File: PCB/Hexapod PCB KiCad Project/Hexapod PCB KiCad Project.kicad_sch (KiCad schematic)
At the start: 3 parts, among them J1 Male Pin Header 1x3, J2 Power Terminal, U1 DEV-16771

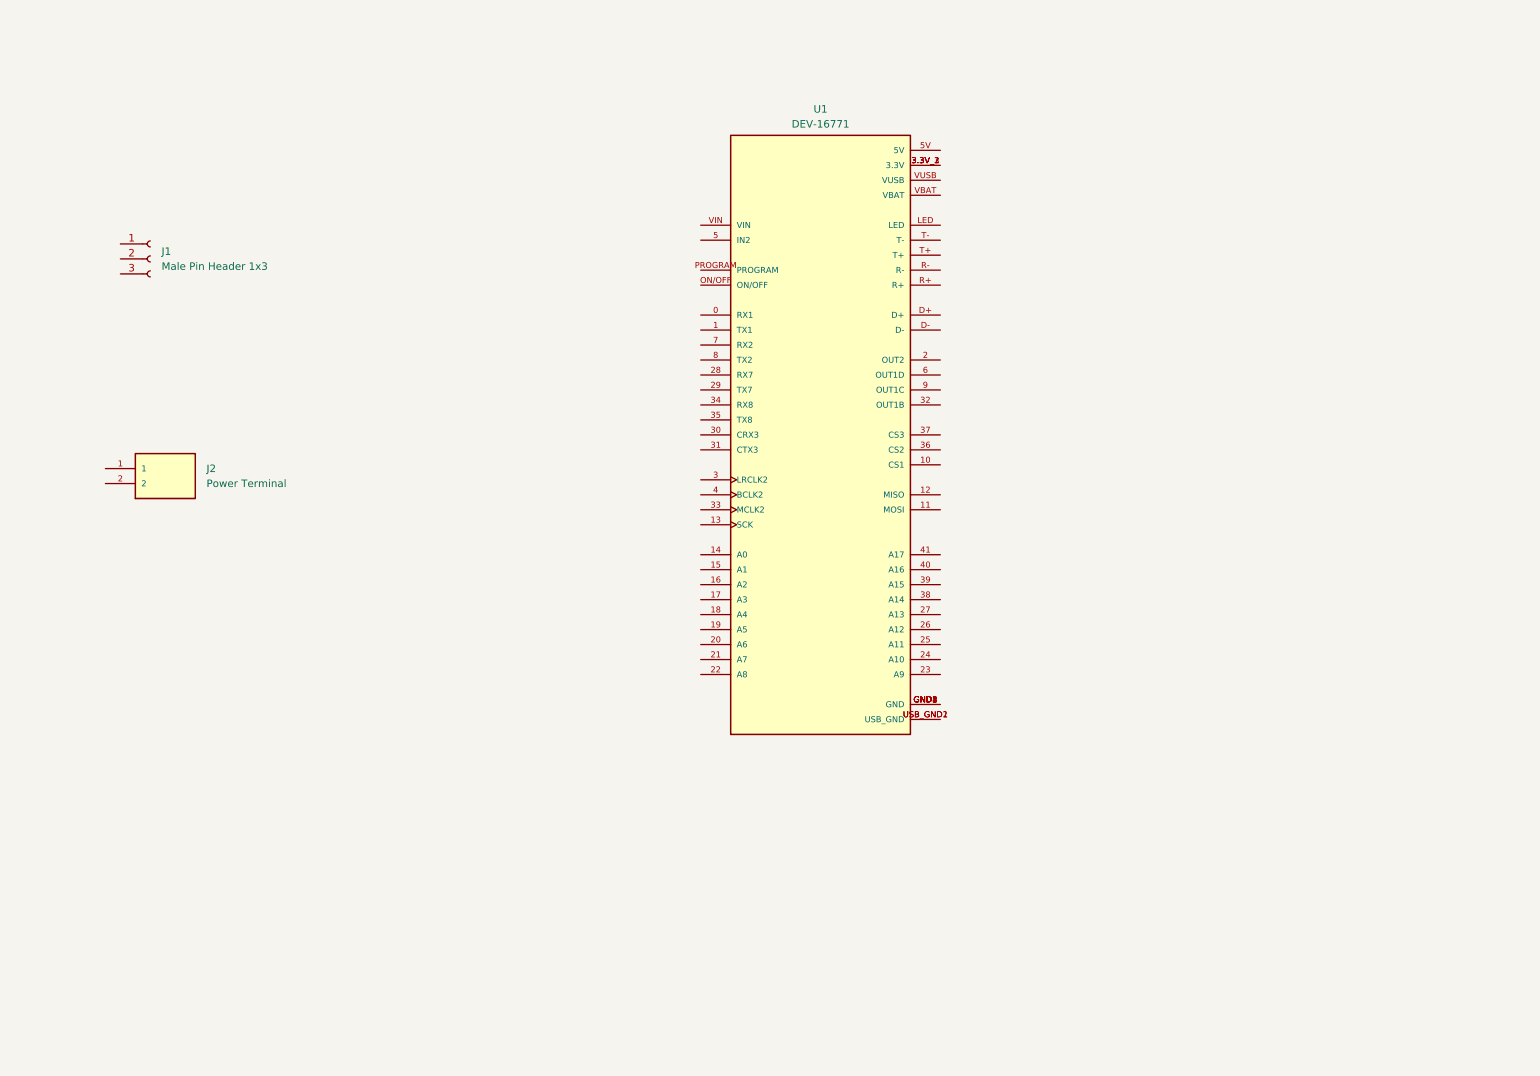
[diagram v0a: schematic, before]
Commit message: Pcb updates
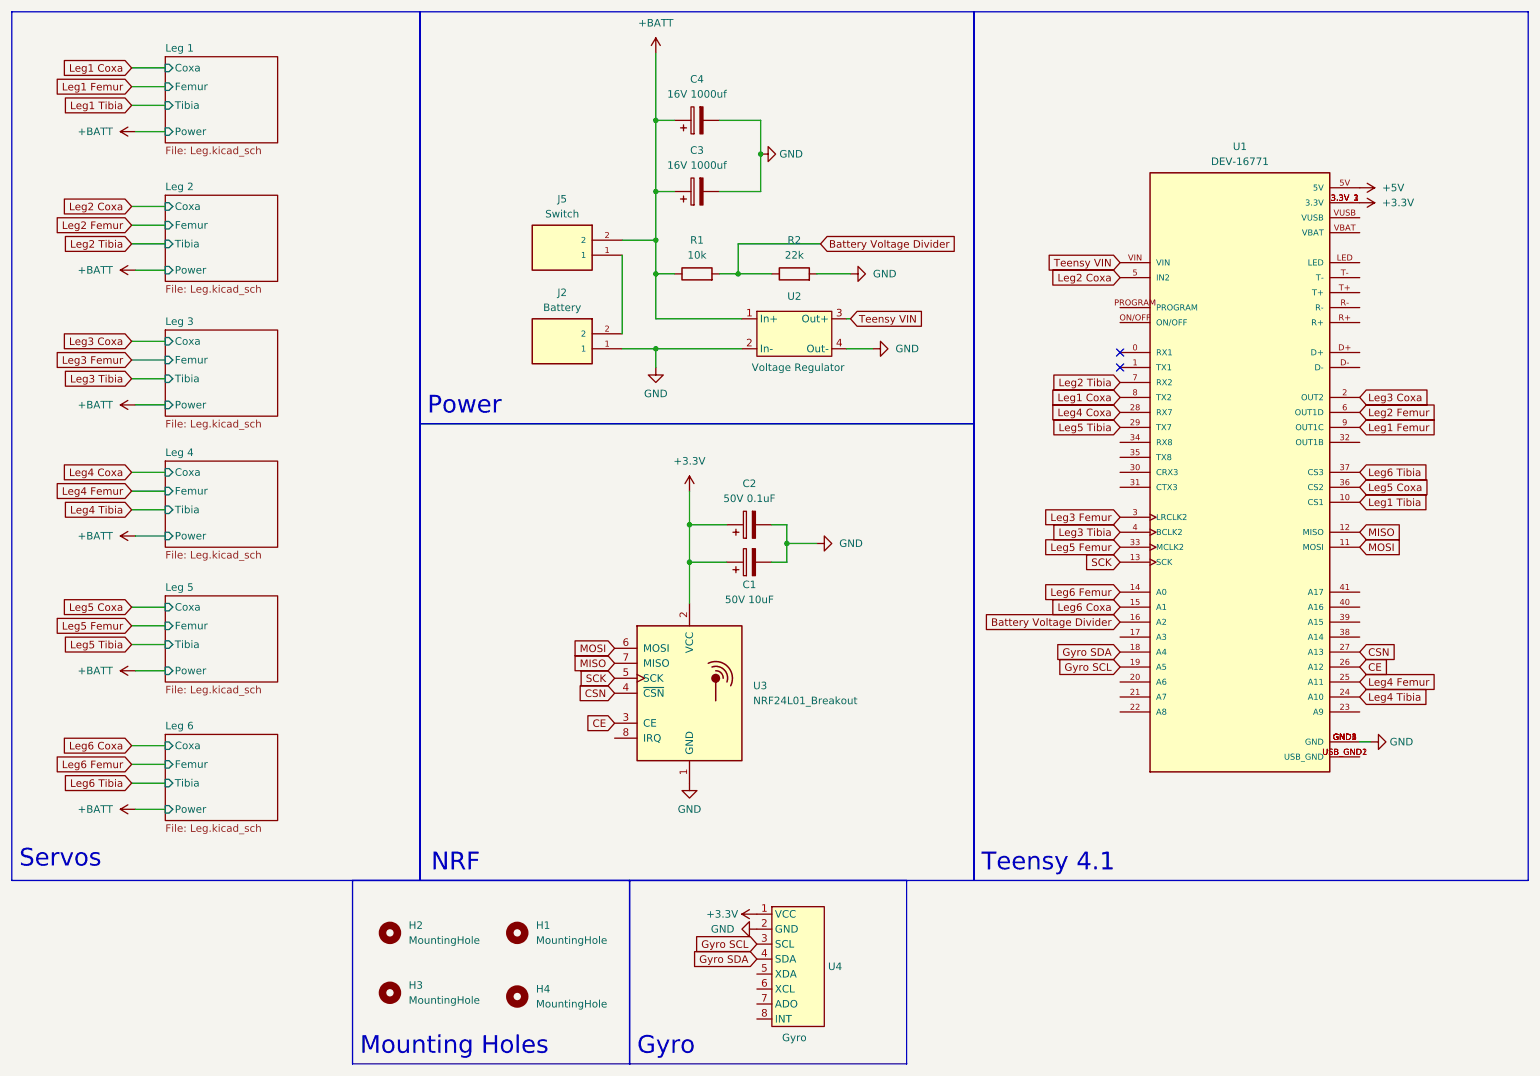
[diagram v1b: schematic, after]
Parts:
- removed J1: Male Pin Header 1x3, Connector_PinHeader_2.54mm:PinHeader_1x03_P2.54mm_Vertical, symbol Connector:Conn_01x03_Socket
- removed J2: Power Terminal, Terminal 2 Pin:CUI_TB005-762-02BE, symbol Terminal 2 Pin:TB005-762-02BE
- removed U1: DEV-16771, TEENSY 4.1:MODULE_DEV-16771, symbol TEENSY 4.1:DEV-16771
- added C1: 50V 10uF, Capacitor_THT:CP_Radial_D5.0mm_P2.00mm, symbol Device:C_Polarized
- added C2: 50V 0.1uF, Capacitor_THT:CP_Radial_D4.0mm_P2.00mm, symbol Device:C_Polarized
- added C3, C4: 16V 1000uf, Capacitor_THT:CP_Radial_D10.0mm_P5.00mm, symbol Device:C_Polarized
- added H1, H2, H3, H4: MountingHole, MountingHole:MountingHole_3.2mm_M3, symbol Mechanical:MountingHole
- added J2: Battery, Terminal 2 Pin:CUI_TB005-762-02BE, symbol Power Terminal 2 Pin:TB005-762-02BE
- added J5: Switch, Terminal 2 Pin:CUI_TB005-762-02BE, symbol Power Terminal 2 Pin:TB005-762-02BE
- added R1: 10k, Resistor_THT:R_Axial_DIN0207_L6.3mm_D2.5mm_P7.62mm_Horizontal, symbol Device:R
- added R2: 22k, Resistor_THT:R_Axial_DIN0207_L6.3mm_D2.5mm_P7.62mm_Horizontal, symbol Device:R
- added U1: DEV-16771, Teensy 4.1:MODULE_DEV-16771, symbol Teensy 4.1:DEV-16771
- added U2: Voltage Regulator, Voltage Regulator LM2596:Voltage Regulator LM2596, symbol Voltage Regulator LM2596:Voltage_Regulator_LM2596
- added U3: NRF24L01_Breakout, RF_Module:nRF24L01_Breakout, symbol RF:NRF24L01_Breakout
- added U4: Gyro, MPU6050 THT:MPU6050 THT, symbol MPU6050 THT:MPU6050_THT
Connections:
- new net: U1.USB_GND1 (USB_GND), U1.USB_GND2 (USB_GND)
- new net: J2.2, J5.1
- new net +3.3V: C1.1, C2.1, U1.3.3V_1 (3.3V), U1.3.3V_2 (3.3V), U1.3.3V_3 (3.3V), U3.2 (VCC), U4.1 (VCC)
- new net +5V: U1.5V
- new net +BATT: C3.1, C4.1, J5.2, R1.1, U2.1 (In+)
- new net Battery Voltage Divider: R1.2, R2.1, U1.16 (A2)
- new net CE: U1.26 (A12), U3.3 (CE)
- new net CSN: U1.27 (A13), U3.4 (~{CSN})
- new net GND: C1.2, C2.2, C3.2, C4.2, J2.1, R2.2, U1.GND1 (GND), U1.GND2 (GND), U1.GND3 (GND), U1.GND4 (GND), U1.GND5 (GND), U2.2 (In-), U2.4 (Out-), U3.1 (GND), U4.2 (GND)
- new net Gyro SCL: U1.19 (A5), U4.3 (SCL)
- new net Gyro SDA: U1.18 (A4), U4.4 (SDA)
- new net Leg1 Coxa: U1.8 (TX2)
- new net Leg1 Femur: U1.9 (OUT1C)
- new net Leg1 Tibia: U1.10 (CS1)
- new net Leg2 Coxa: U1.5 (IN2)
- new net Leg2 Femur: U1.6 (OUT1D)
- new net Leg2 Tibia: U1.7 (RX2)
- new net Leg3 Coxa: U1.2 (OUT2)
- new net Leg3 Femur: U1.3 (LRCLK2)
- new net Leg3 Tibia: U1.4 (BCLK2)
- new net Leg4 Coxa: U1.28 (RX7)
- new net Leg4 Femur: U1.25 (A11)
- new net Leg4 Tibia: U1.24 (A10)
- new net Leg5 Coxa: U1.36 (CS2)
- new net Leg5 Femur: U1.33 (MCLK2)
- new net Leg5 Tibia: U1.29 (TX7)
- new net Leg6 Coxa: U1.15 (A1)
- new net Leg6 Femur: U1.14 (A0)
- new net Leg6 Tibia: U1.37 (CS3)
- new net MISO: U1.12 (MISO), U3.7 (MISO)
- new net MOSI: U1.11 (MOSI), U3.6 (MOSI)
- new net SCK: U1.13 (SCK), U3.5 (SCK)
- new net Teensy VIN: U1.VIN, U2.3 (Out+)
- no-connect marks 0 -> 2
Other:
- added sheet Leg 1 (Leg.kicad_sch)
- added sheet Leg 2 (Leg.kicad_sch)
- added sheet Leg 3 (Leg.kicad_sch)
- added sheet Leg 4 (Leg.kicad_sch)
- added sheet Leg 5 (Leg.kicad_sch)
- added sheet Leg 6 (Leg.kicad_sch)
- note added: "Gyro"
- note added: "Mounting Holes"
- note added: "NRF"
- note added: "Power"
- note added: "Servos"
- note added: "Teensy 4.1"
